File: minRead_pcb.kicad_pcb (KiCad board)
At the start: 2 copper layers, 62.4 x 115 mm, 111 parts, among them J1 USB_C_Receptacle, J2 FH34SRJ-24S-0.5SH_50_, J3 FH34SRJ-6S-0.5SH_50_, J5 Conn_01x02, J7 Micro_SD_Card, Q10 BSS138, Q11 BSS138, Q16 MMBT3906, Q17 MMBT3904, Q18 AO3419, Q4 [BSS138] AO3400A, Q5 AO3419, Q6 AO3419, SW1 SW_Push, SW10 SW_Push, SW11 SW_Push, SW2 SW_Push, SW3 SW_Push, SW4 SW_Push, SW6 SW_Push, SW8 SW_Push, SW9 SW_Push, U1 TPD4E1U06DBVR, U11 AP3031KTR, U3 AP2112K-3.3, U4 ESP32-S3-WROOM-1, U6 TPD4E1U06DBVR, U7 MCP73832-2-OT

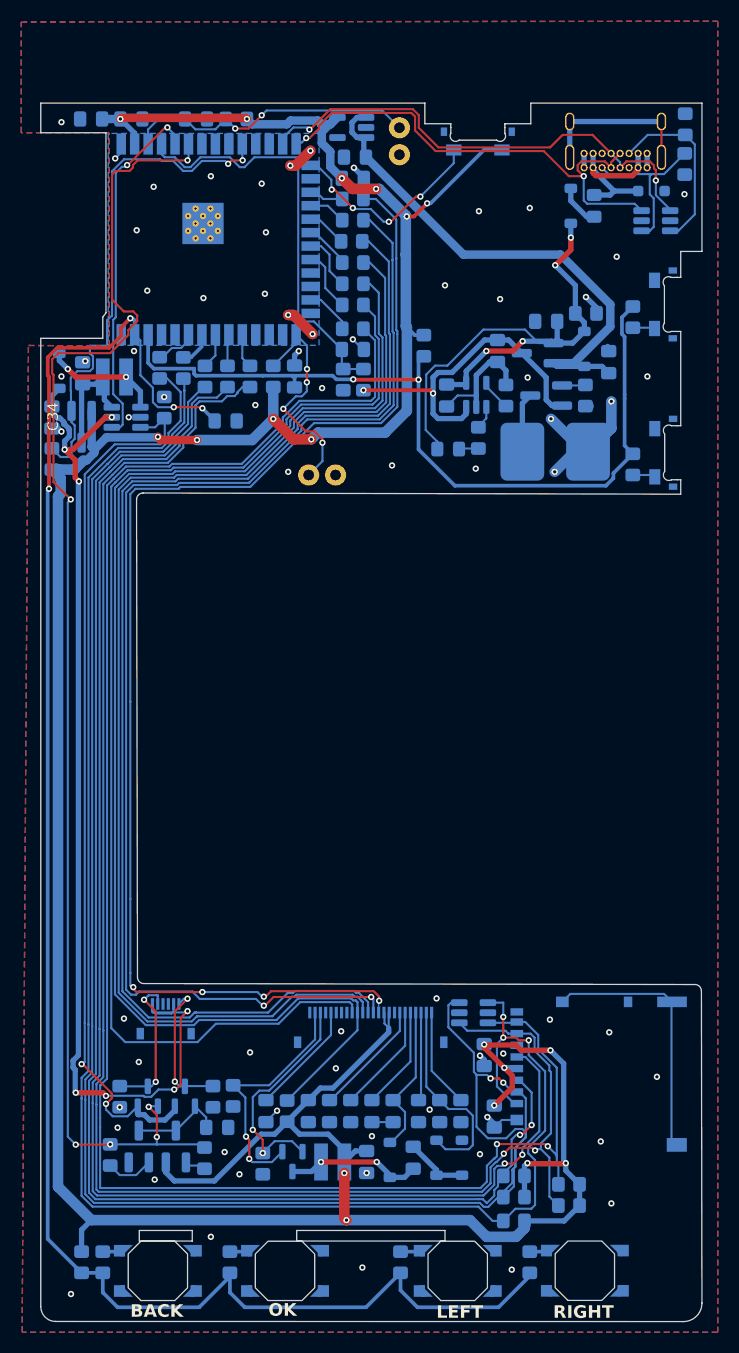
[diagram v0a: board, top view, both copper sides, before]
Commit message: switch to 5k1 prog
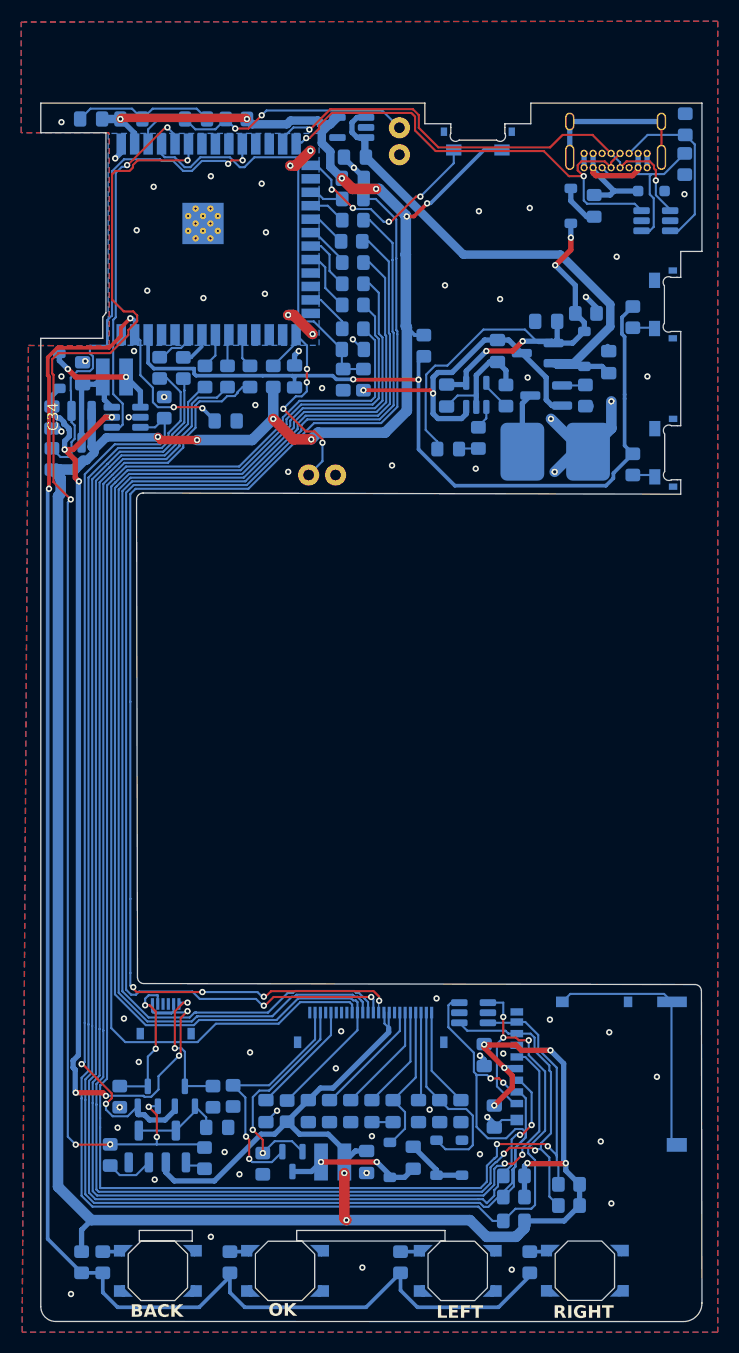
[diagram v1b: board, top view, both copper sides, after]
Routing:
- net B-: track 92.4 -> 107.3 mm
- net LDO_IN: track 49.3 -> 51.1 mm
- net LED_SW: track 99.9 -> 98.9 mm
